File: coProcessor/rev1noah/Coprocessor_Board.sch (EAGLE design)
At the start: 98 parts, among them IC1 STM32F405RGT6, J1 USB_MINI-B_SMT, J4 30320-6002HB, J5 5008730806, P1 39-30-08, Q1 L78M05CV

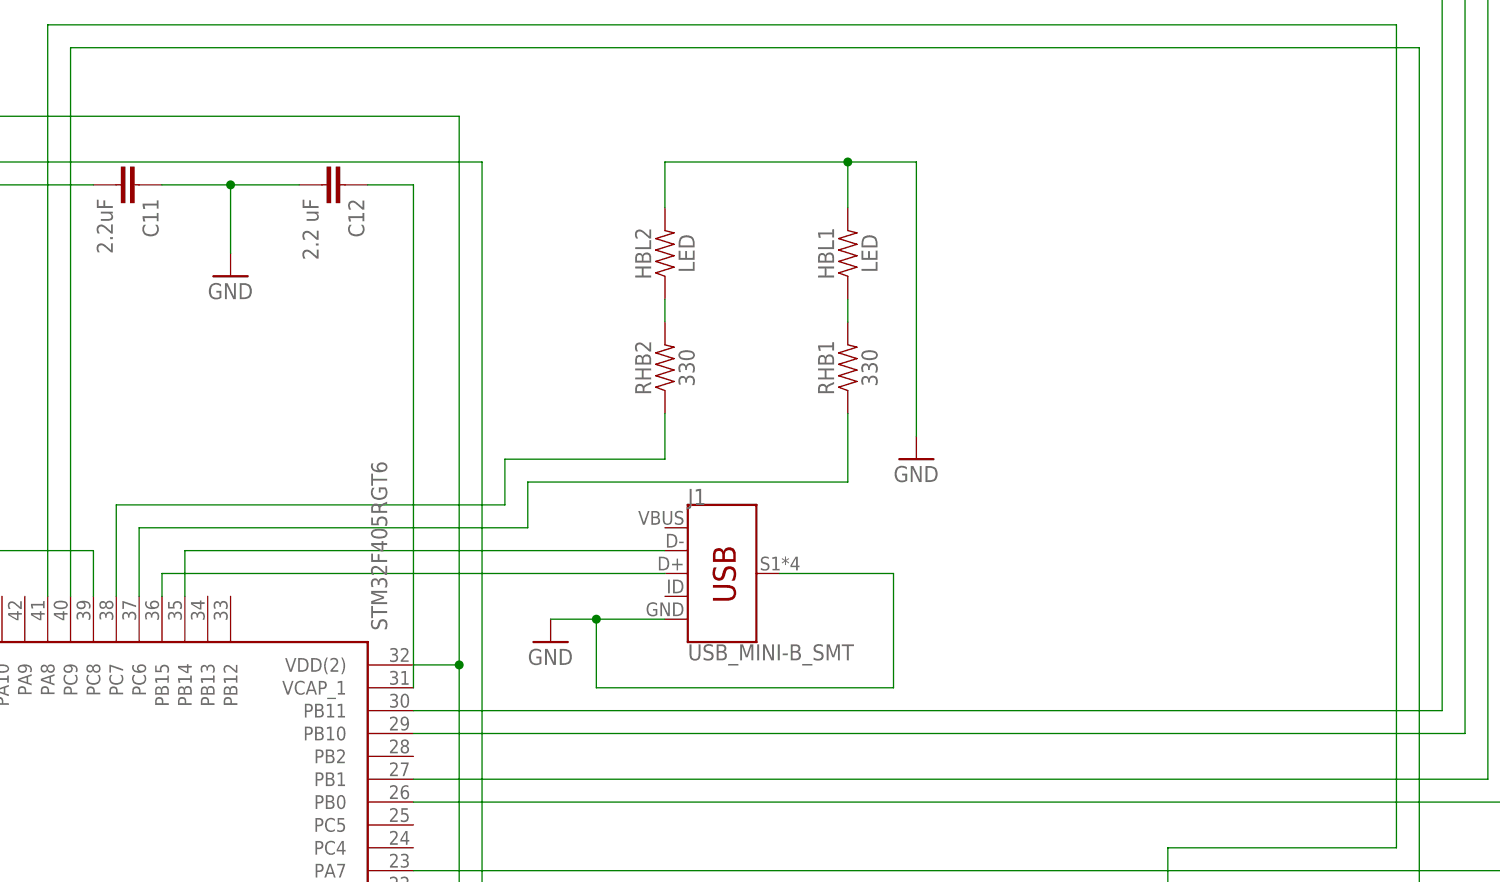
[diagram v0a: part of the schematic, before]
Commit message: Fixing USB lines, we RF now boyz
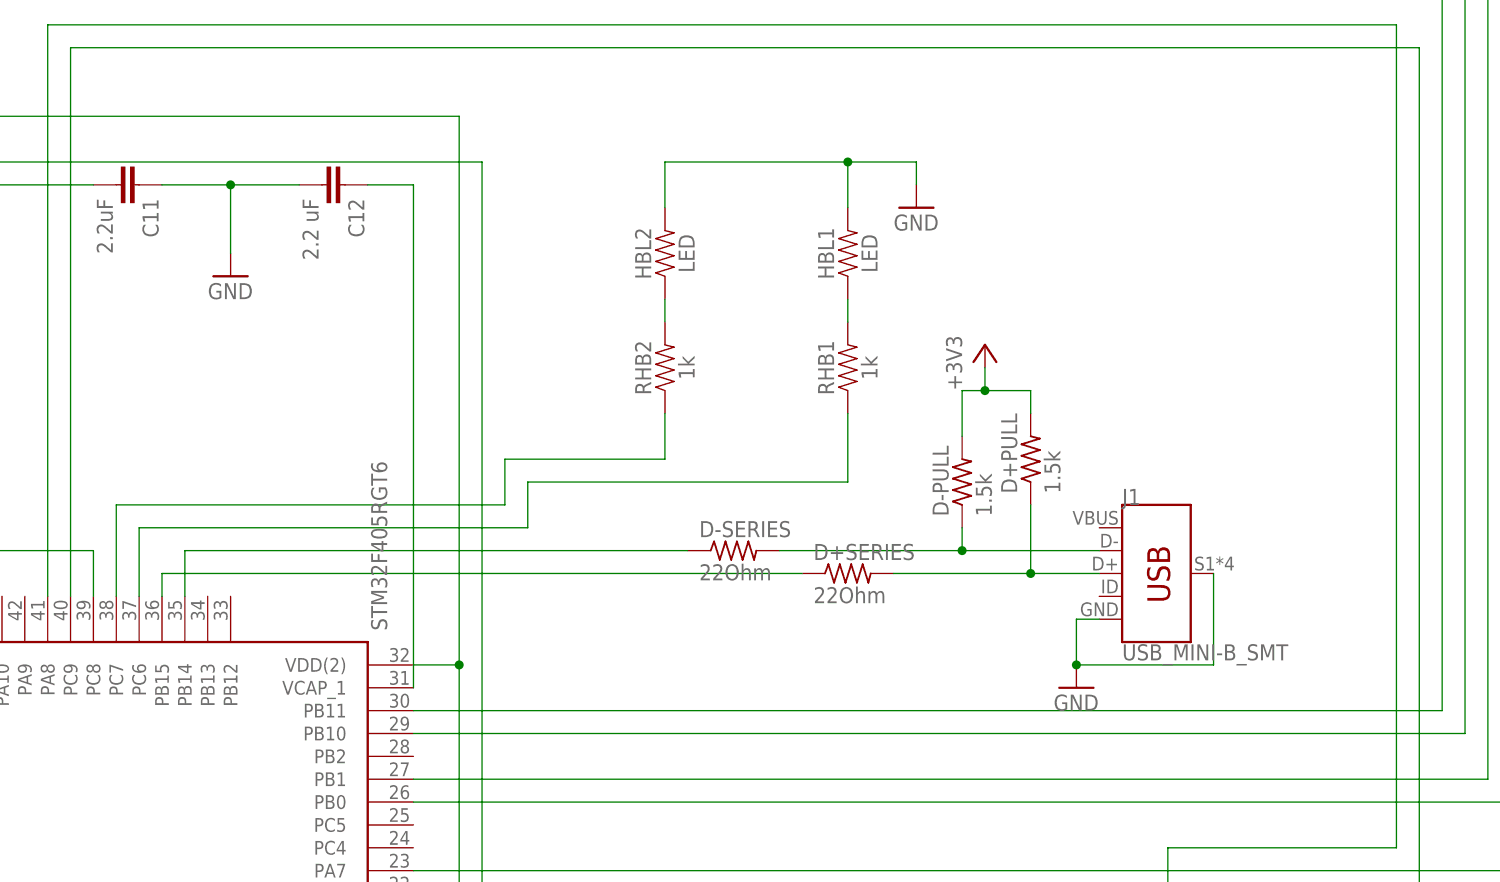
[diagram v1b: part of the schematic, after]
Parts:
- added D+PULL, D-PULL: 1.5k, resistor:R-US_0204/7
- added D+SERIES, D-SERIES: 22Ohm, resistor:R-US_0204/7
- RHB1: value 330 -> 1k; device SparkFun-Resistors:1KOHM-VERT-1/4W-1% -> SparkFun-Resistors:1KOHM-HORIZ-1/4W-1%
- RHB2: value 330 -> 1k; device SparkFun-Resistors:1KOHM-VERT-1/4W-1% -> SparkFun-Resistors:1KOHM-HORIZ-1/4W-5%
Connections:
- new net D+CON: D+PULL.1, D+SERIES.2, J1.D+
- new net D-CON: D-PULL.1, D-SERIES.2, J1.D-
- net 3.3V: now also D+PULL.2, D-PULL.2
- net USB_OTG_HS_DM: now also D-SERIES.1; no longer J1.D-
- net USB_OTG_HS_DP: now also D+SERIES.1; no longer J1.D+
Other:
- moved on the sheet: J1
